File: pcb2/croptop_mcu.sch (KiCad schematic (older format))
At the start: 95 parts, among them J1 TSM-106-01-L-SV, J2 0473460001, J3 87583-2010BLF, Q1 BSS138, Q2 BSS84, SW1 SW_Push, U1 PIC32MX795F512L, U2 REG71055DDC, U3 AP22802AW5, U4 TPS61169DCK, U5 TPS62131RGT, U6 TPS70950DBV, U7 TPD4E1U06DBV, Y1 ABLS-8.000MHZ-B4-T

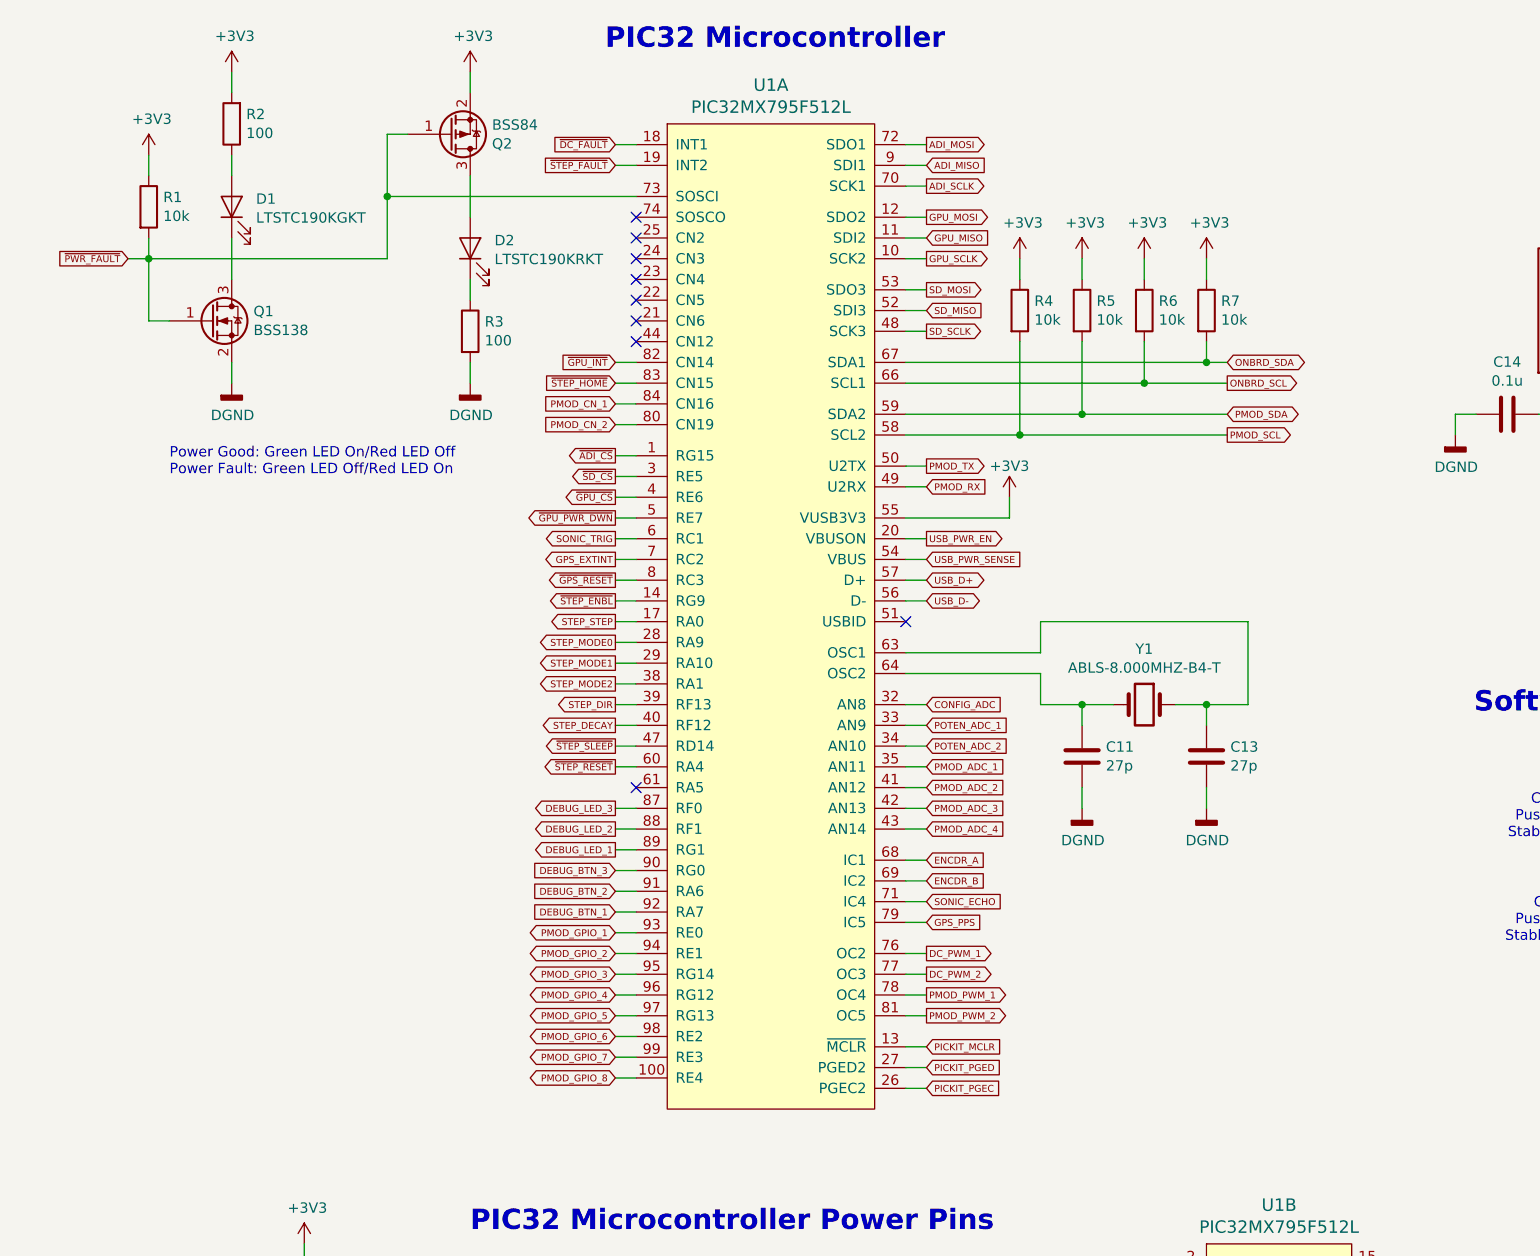
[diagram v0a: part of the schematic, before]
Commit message: Finished PCB
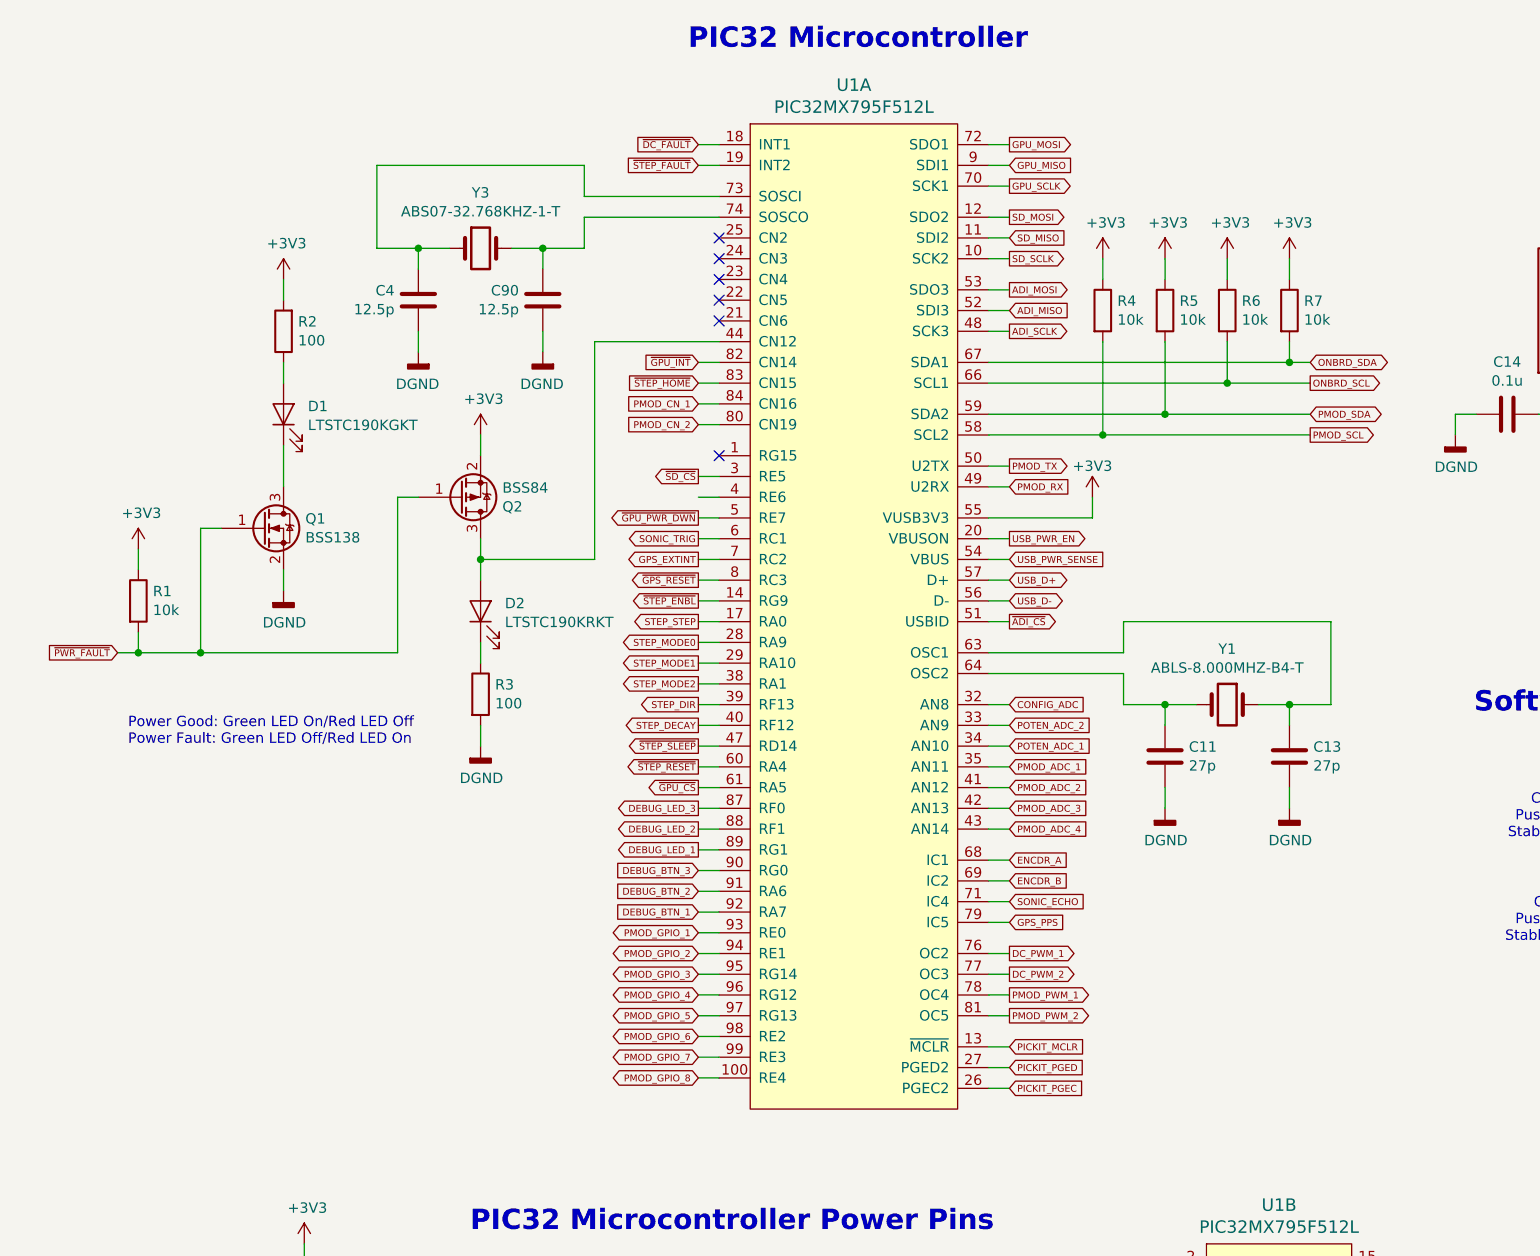
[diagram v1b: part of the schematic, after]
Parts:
- added C4, C90: 12.5p, Capacitor_SMD:C_0402_1005Metric, symbol Device:C
- added Y3: ABS07-32.768KHZ-1-T, croptop:ABLS_SEC, symbol Device:Crystal
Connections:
- net ADI_MISO: now also U1.52 (SDI3); no longer U1.9 (SDI1)
- net ADI_MOSI: now also U1.53 (SDO3); no longer U1.72 (SDO1)
- net ADI_SCLK: now also U1.48 (SCK3); no longer U1.70 (SCK1)
- net DGND: now also C4.2, C90.2
- net GPU_MISO: now also U1.9 (SDI1); no longer U1.11 (SDI2)
- net GPU_MOSI: now also U1.72 (SDO1); no longer U1.12 (SDO2)
- net GPU_SCLK: now also U1.70 (SCK1); no longer U1.10 (SCK2)
- net POTEN_ADC_1: now also U1.34 (AN10); no longer U1.33 (AN9)
- net POTEN_ADC_2: now also U1.33 (AN9); no longer U1.34 (AN10)
- net SD_MISO: now also U1.11 (SDI2); no longer U1.52 (SDI3)
- net SD_MOSI: now also U1.12 (SDO2); no longer U1.53 (SDO3)
- net SD_SCLK: now also U1.10 (SCK2); no longer U1.48 (SCK3)
- net ~ADI_CS: now also U1.51 (USBID); no longer U1.1 (RG15)
- net ~GPU_CS: now also U1.61 (RA5); no longer U1.4 (RE6)
- net ~PWR_FAULT: no longer U1.73 (SOSCI)
- net at U1.44 (CN12): now also D2.2 (A), Q2.3 (D)
- net at U1.74 (SOSCO): now also C90.1, Y3.2
- new net: C4.1, U1.73 (SOSCI), Y3.1
- no-connect marks 17 -> 14
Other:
- moved on the sheet: C11, C13, D1, D2, Q1, Q2, R1, R2, R3, R4, R5, R6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
